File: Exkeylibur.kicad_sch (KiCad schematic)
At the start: 23 parts, among them SW1 SW_Push, SW10 SW_Push, SW11 SW_Push, SW12 SW_Push, SW13 SW_Push, SW14 SW_Push, SW15 SW_Push, SW16 SW_Push, SW17 SW_Push, SW18 SW_Push, SW2 SW_Push, SW3 SW_Push, SW4 SW_Push, SW5 SW_Push, SW6 SW_Push, SW7 SW_Push, SW8 SW_Push, SW9 SW_Push, U1 ProMicro

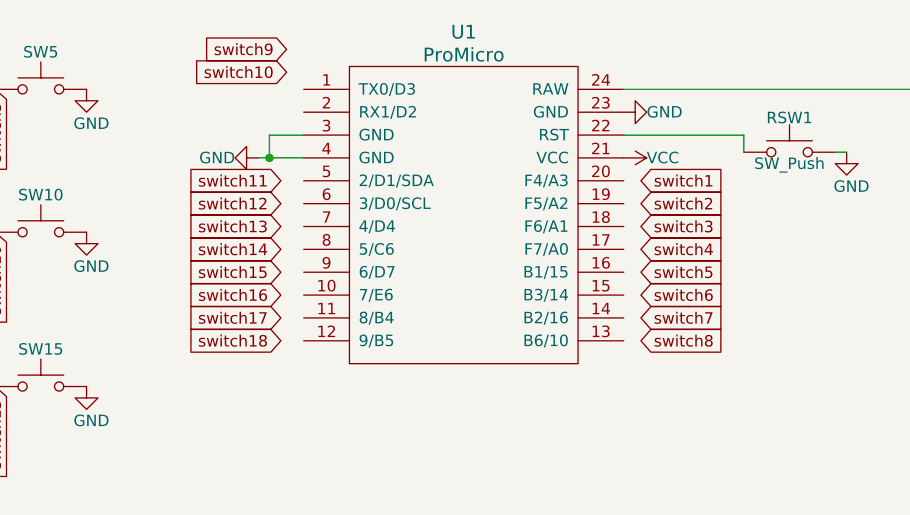
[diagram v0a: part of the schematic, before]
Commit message: backannotate to schematic:
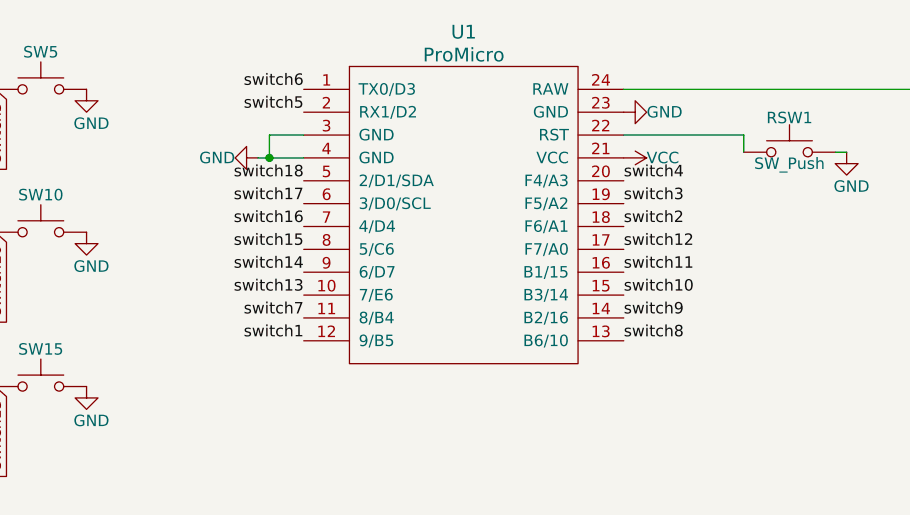
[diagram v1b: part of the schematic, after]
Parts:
- BT_GND1: footprint (none) -> Exkeylibur:bat_gnd_mountingHole
- BT_V1: footprint (none) -> Exkeylibur:Bat_MountingHole
- PWR_SW1: footprint Exkeylibur:keyboard_power_switch -> Kailh:SPDT_C128955
- SW10, SW11, SW12, SW13, SW14, SW15, SW16, SW17, SW18, SW2, SW3, SW4, SW5, SW6, SW7, SW8, SW9: footprint (none) -> Exkeylibur:choc_switch_reversible
- U1: footprint Exkeylibur:ProMicro_v3_min -> kbd:ProMicro_v3_min
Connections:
- net switch1: now also U1.12 (9/B5)
- net switch10: now also U1.15 (B3/14)
- net switch11: now also U1.16 (B1/15)
- net switch12: now also U1.17 (F7/A0)
- net switch13: now also U1.10 (7/E6)
- net switch14: now also U1.9 (6/D7)
- net switch15: now also U1.8 (5/C6)
- net switch16: now also U1.7 (4/D4)
- net switch17: now also U1.6 (3/D0/SCL)
- net switch18: now also U1.5 (2/D1/SDA)
- net switch2: now also U1.18 (F6/A1)
- net switch3: now also U1.19 (F5/A2)
- net switch4: now also U1.20 (F4/A3)
- net switch5: now also U1.2 (RX1/D2)
- net switch6: now also U1.1 (TX0/D3)
- net switch7: now also U1.11 (8/B4)
- net switch8: now also U1.13 (B6/10)
- net switch9: now also U1.14 (B2/16)
